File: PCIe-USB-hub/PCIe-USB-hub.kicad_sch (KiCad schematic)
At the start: 1 part, among them J1 PCIexpress_x1

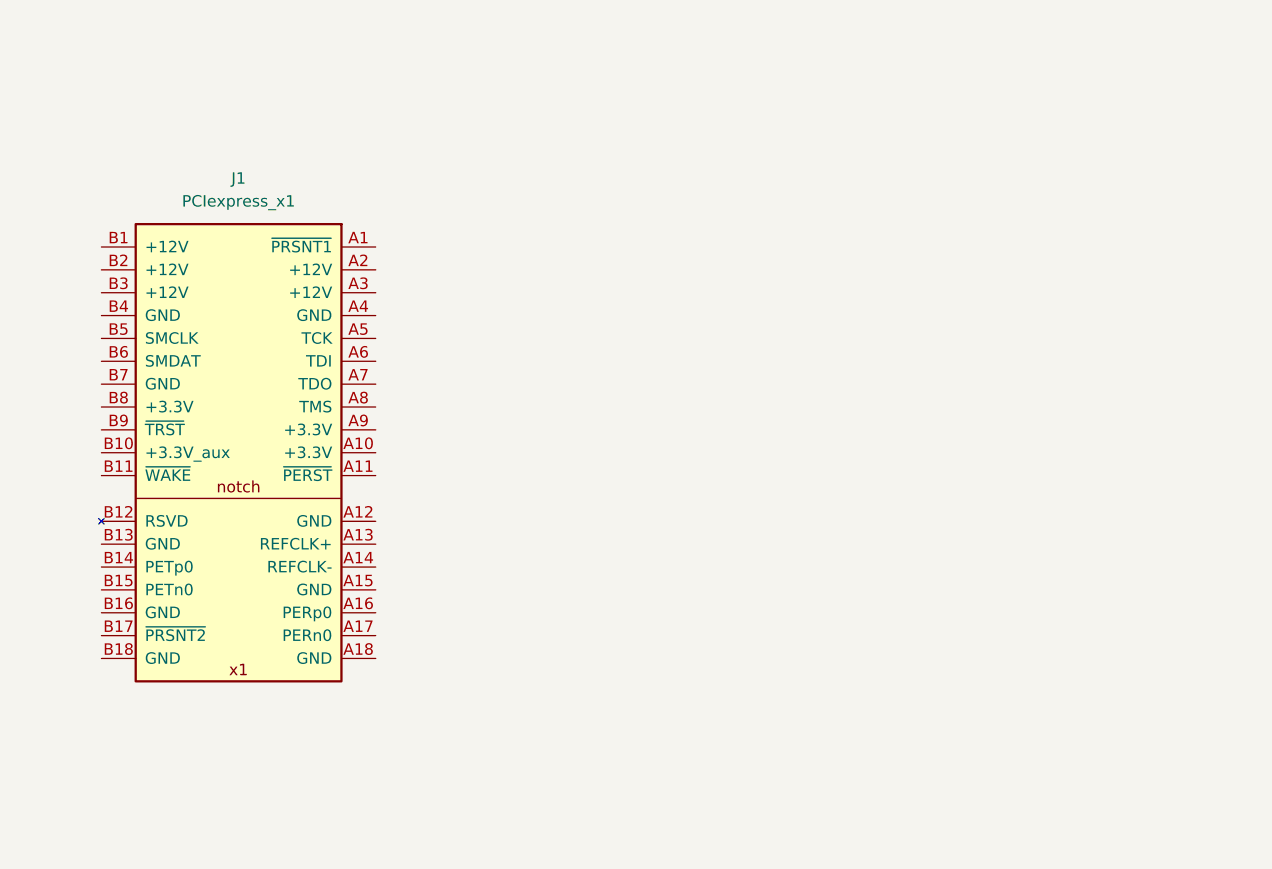
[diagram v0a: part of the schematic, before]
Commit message: Частично добавил компоненты
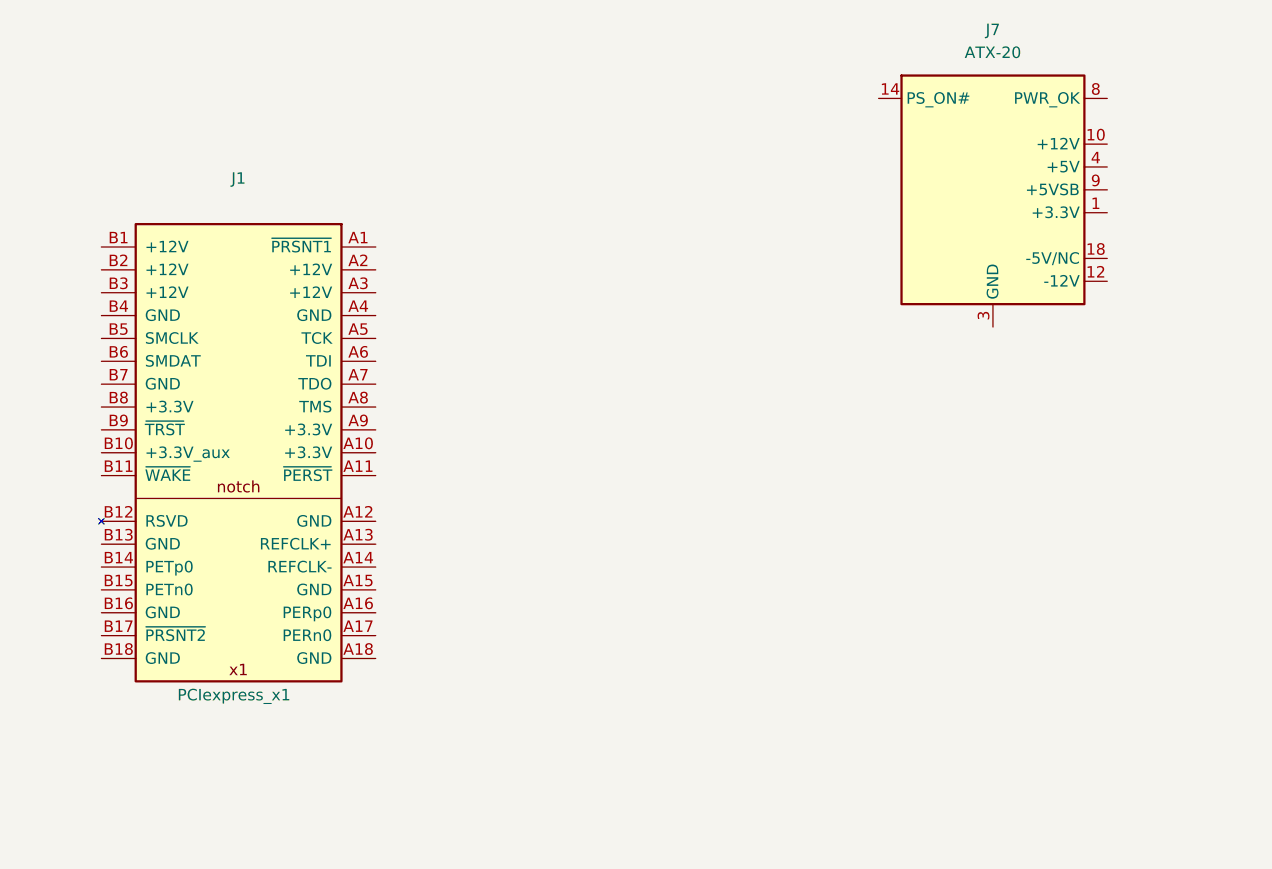
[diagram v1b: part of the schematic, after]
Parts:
- added J7: ATX-20, symbol Connector:ATX-20
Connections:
- new net: J7.1 (+3.3V), J7.11 (+3.3V), J7.2 (+3.3V)
- new net: J7.13 (GND), J7.15 (GND), J7.16 (GND), J7.17 (GND), J7.3 (GND), J7.5 (GND), J7.7 (GND)
- new net: J7.19 (+5V), J7.20 (+5V), J7.4 (+5V), J7.6 (+5V)
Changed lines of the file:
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@@
 	(paper "A3")
+	(symbol
+		(lib_id "Connector:ATX-20")
+		(at 257.81 77.47 0)
+		(unit 1)
+		(exclude_from_sim no)
+		(in_bom yes)
+		(on_board yes)
+		(dnp no)
+		(fields_autoplaced yes)
+		(property "Reference" "J7"
+			(at 257.81 59.69 0)
+			(effects
+				(font
+					(size 1.27 1.27)
+				)
+			)
+		)
+		(property "Value" "ATX-20"
+			(at 257.81 62.23 0)
+			(effects
+				(font
+					(size 1.27 1.27)
+				)
+			)
+		)
+		(property "Footprint" ""
+			(at 257.81 80.01 0)
+			(effects
+				(font
+					(size 1.27 1.27)
+				)
+				(hide yes)
+			)
+		)
+		(property "Datasheet" "https://web.aub.edu.lb/pub/docs/atx_201.pdf#page=20"
+			(at 285.75 91.44 0)
+			(effects
+				(font
+					(size 1.27 1.27)
+				)
+				(hide yes)
+			)
+		)
+		(property "Description" "ATX Power supply 20pins"
+			(at 257.81 77.47 0)
+			(effects
+				(font
+					(size 1.27 1.27)
+				)
+				(hide yes)
+			)
+		)
+		(pin "11"
+		)
+		(pin "8"
+		)
+		(pin "9"
+		)
+		(pin "15"
+		)
+		(pin "16"
+		)
+		(pin "5"
+		)
+		(pin "10"
+		)
+		(pin "19"
+		)
+		(pin "3"
+		)
+		(pin "6"
+		)
+		(pin "1"
+		)
+		(pin "14"
+		)
+		(pin "13"
+		)
+		(pin "17"
+		)
+		(pin "7"
+		)
+		(pin "4"
+		)
+		(pin "20"
+		)
+		(pin "18"
+		)
+		(pin "2"
+		)
+		(pin "12"
+		)
+		(instances
+			(project ""
+				(path "/9ca96bdf-018d-455b-a724-78a2bbb0adec"
+					(reference "J7")
+					(unit 1)
+				)
+			)
+		)
+	)
 	(symbol
 		(lib_id "PCIexpress:PCIexpress_x1")
@@
 		(on_board yes)
 		(dnp no)
-		(fields_autoplaced yes)
 		(property "Reference" "J1"
 			(at 173.99 76.2 0)
@@
 		)
 		(property "Value" "PCIexpress_x1"
-			(at 173.99 78.74 0)
+			(at 173.482 133.604 0)
 			(effects
 				(font
